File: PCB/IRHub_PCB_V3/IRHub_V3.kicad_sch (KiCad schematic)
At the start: 66 parts, among them J2 USB_C_Receptacle_USB2.0_16P, Q1 UMH3N, Q2 AO3400A, Q3 AO3400A, U1 ESP-12F, U2 CH340C, U3 AMS1117-3.3, U4 TSOP382xx, U5 ME6211C33M5

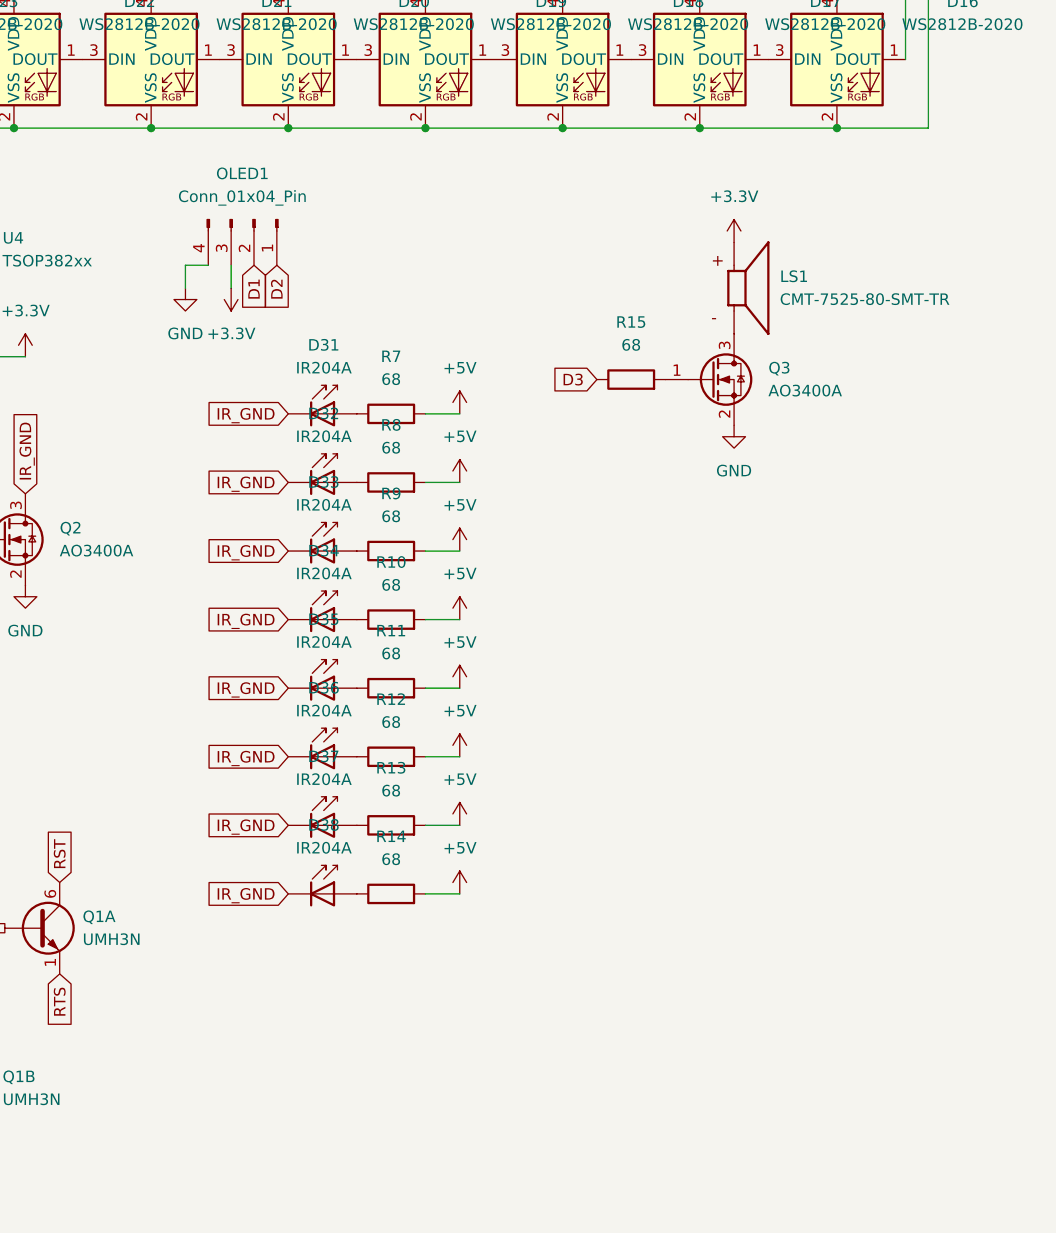
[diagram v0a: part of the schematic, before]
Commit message: complete schematic i think ?
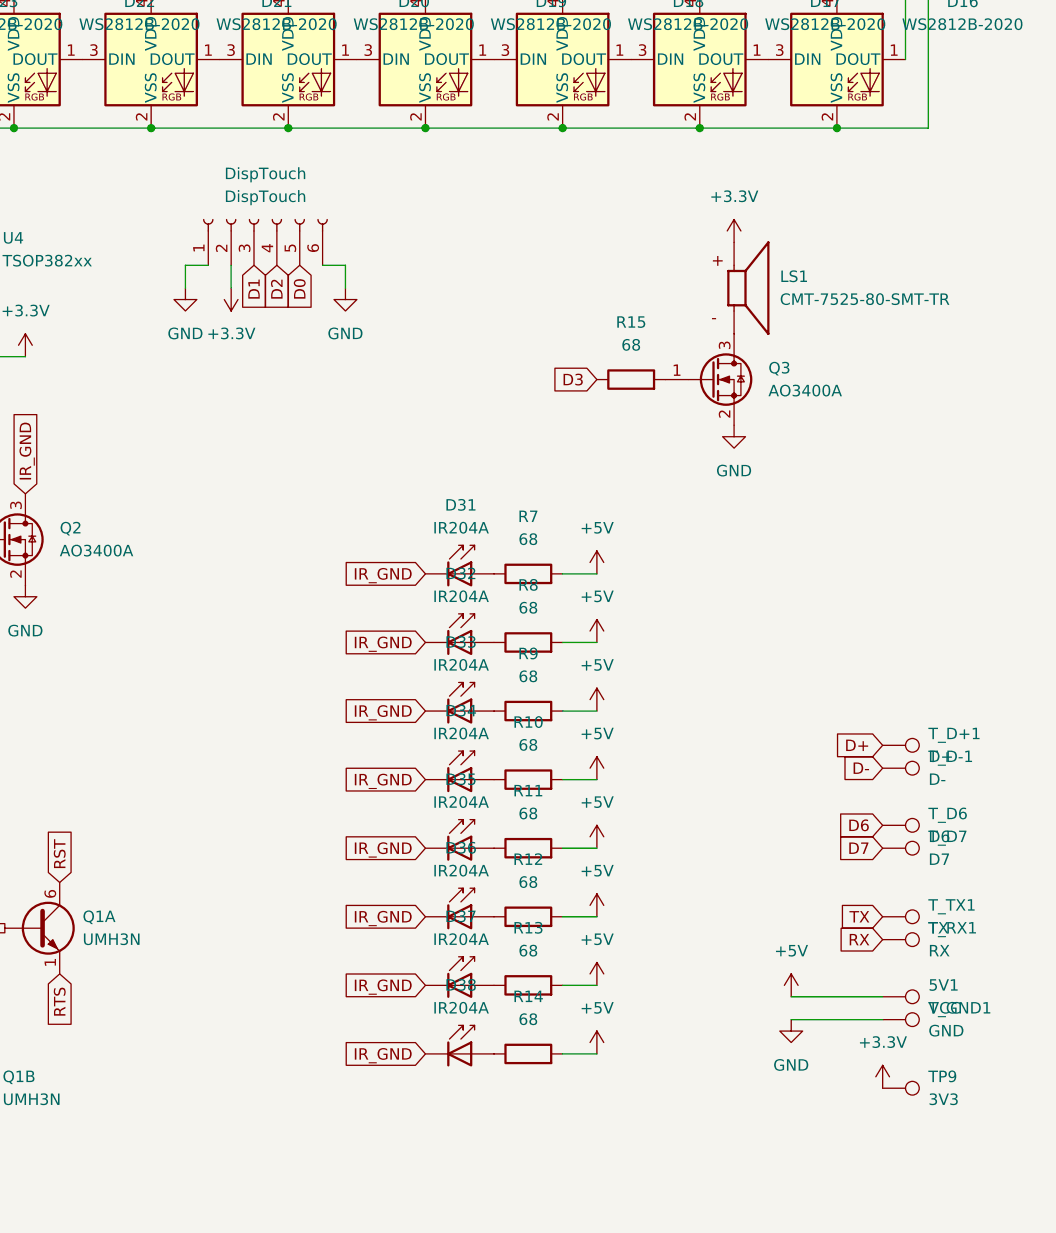
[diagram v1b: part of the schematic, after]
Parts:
- removed OLED1: Conn_01x04_Pin, Connector_PinHeader_2.54mm:PinHeader_1x04_P2.54mm_Vertical, symbol Connector:Conn_01x04_Pin
- added 5V1: VCC, TestPoint:TestPoint_Pad_D2.0mm, symbol Connector:TestPoint
- added DispTouch: DispTouch, Connector_JST:JST_SH_BM06B-SRSS-TB_1x06-1MP_P1.00mm_Vertical, symbol Connector:Conn_01x06_Socket
- added TP9: 3V3, TestPoint:TestPoint_Pad_D2.0mm, symbol Connector:TestPoint
- added T_D+1: D+, TestPoint:TestPoint_Pad_D2.0mm, symbol Connector:TestPoint
- added T_D-1: D-, TestPoint:TestPoint_Pad_D2.0mm, symbol Connector:TestPoint
- added T_D6: D6, TestPoint:TestPoint_Pad_D2.0mm, symbol Connector:TestPoint
- added T_D7: D7, TestPoint:TestPoint_Pad_D2.0mm, symbol Connector:TestPoint
- added T_GND1: GND, TestPoint:TestPoint_Pad_D2.0mm, symbol Connector:TestPoint
- added T_RX1: RX, TestPoint:TestPoint_Pad_D2.0mm, symbol Connector:TestPoint
- added T_TX1: TX, TestPoint:TestPoint_Pad_D2.0mm, symbol Connector:TestPoint
- LS1: footprint CMT-7525-80-SMT-TR:XDCR_CMT-7525-80-SMT-TR -> CMT-7525:XDCR_CMT-7525-80-SMT-TR
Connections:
- net +3.3V: now also DispTouch.2 (Pin_2), TP9.1
- net +5V: now also 5V1.1
- net D+: now also T_D+1.1
- net D-: now also T_D-1.1
- net D0: now also DispTouch.5 (Pin_5)
- net D1: now also DispTouch.3 (Pin_3)
- net D2: now also DispTouch.4 (Pin_4)
- net D6: now also T_D6.1
- net D7: now also T_D7.1
- net GND: now also DispTouch.1 (Pin_1), DispTouch.6 (Pin_6), T_GND1.1
- net RX: now also T_RX1.1
- net TX: now also T_TX1.1
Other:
- moved on the sheet: D31, D32, D33, D34, D35, D36, D37, D38, R10, R11, R12, R13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

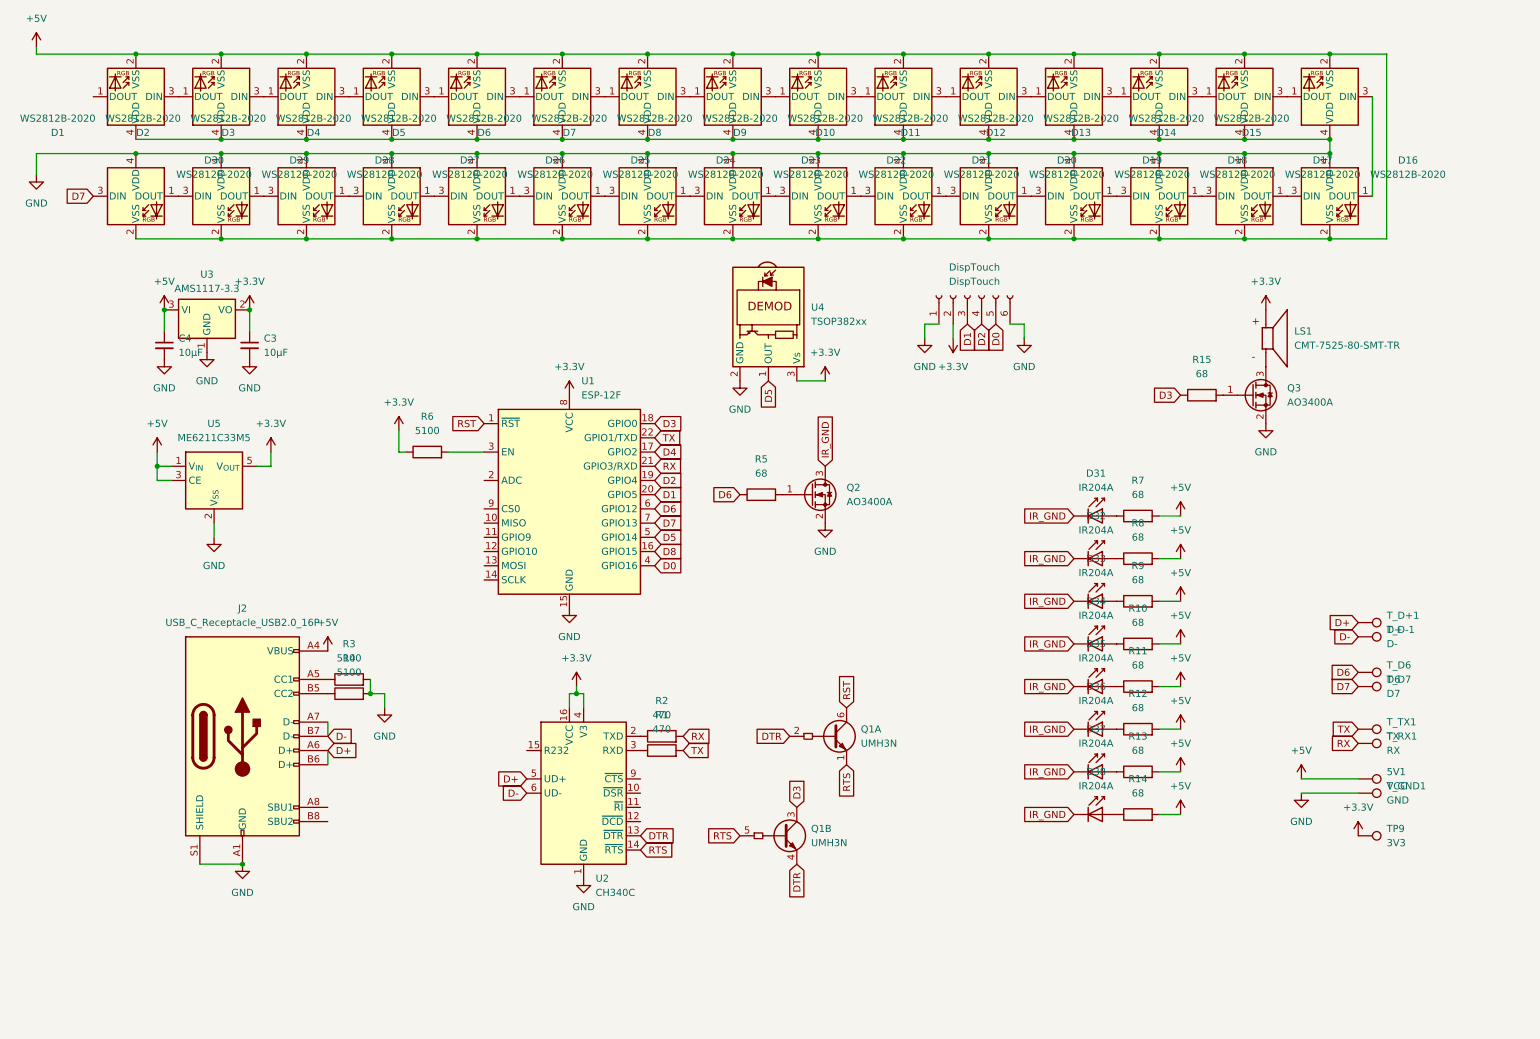
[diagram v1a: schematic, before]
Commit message: final design i think
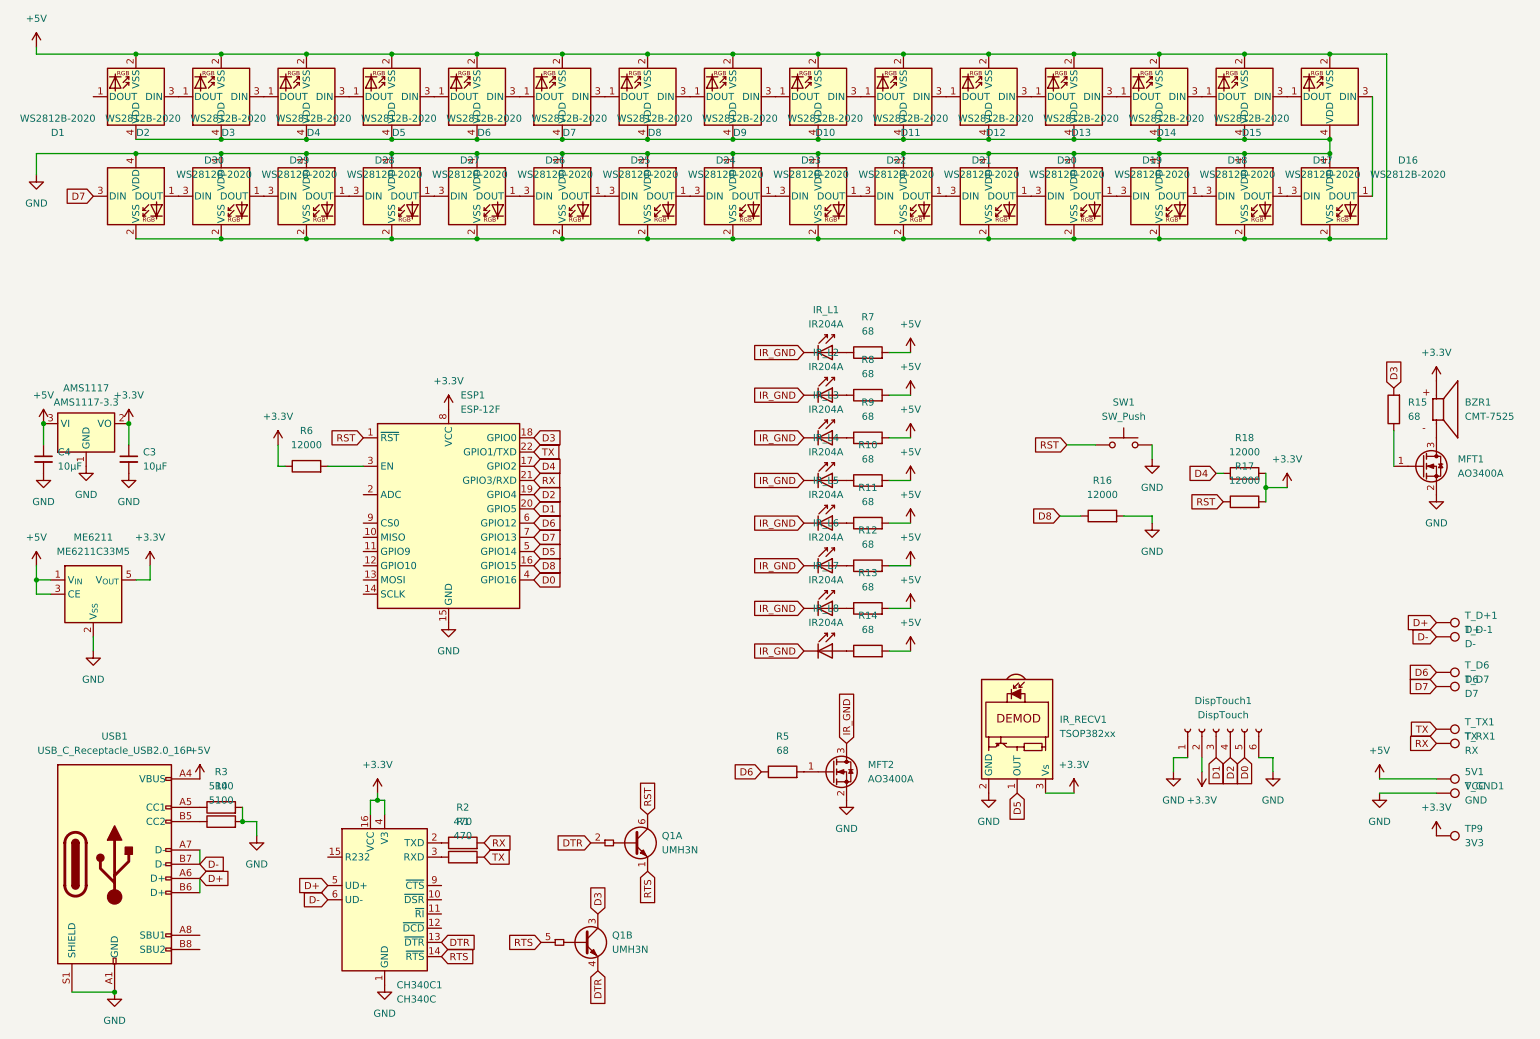
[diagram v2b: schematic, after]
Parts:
- removed D32, D33, D34, D35, D36, D37, D38: IR204A, LED_THT:LED_D3.0mm_IRBlack, symbol LED:IR204A
- added IR_L2, IR_L3, IR_L4, IR_L5, IR_L6, IR_L7, IR_L8: IR204A, LED_THT:LED_D3.0mm_IRBlack, symbol LED:IR204A
- added R16, R17, R18: 12000, Resistor_SMD:R_1206_3216Metric_Pad1.30x1.75mm_HandSolder, symbol Device:R
- added SW1: SW_Push, Button_Switch_SMD:SW_SPST_TS-1088-xR020, symbol Switch:SW_Push
- BZR1: renamed from LS1; value CMT-7525-80-SMT-TR -> CMT-7525
- R6: value 5100 -> 12000
- renumbered U3 to AMS1117, U2 to CH340C1, DispTouch to DispTouch1, U1 to ESP1, D31 to IR_L1, U4 to IR_RECV1, U5 to ME6211, Q3 to MFT1, Q2 to MFT2, J2 to USB1
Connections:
- net +3.3V: now also R17.2, R18.2
- net D3: now also R15.2; no longer R15.1
- net D4: now also R18.1
- net D8: now also R16.1
- net GND: now also R16.2, SW1.2
- net IR_GND: now also IR_L2.1 (K), IR_L3.1 (K), IR_L4.1 (K), IR_L5.1 (K), IR_L6.1 (K), IR_L7.1 (K), IR_L8.1 (K)
- net RST: now also R17.1, SW1.1
- net at R13.1: now also IR_L7.2 (A)
- net at R8.1: now also IR_L2.2 (A)
- net at R11.1: now also IR_L5.2 (A)
- net at R10.1: now also IR_L4.2 (A)
- net at R9.1: now also IR_L3.2 (A)
- net at MFT1.1 (G): now also R15.1; no longer R15.2
- net at R12.1: now also IR_L6.2 (A)
- net at R14.1: now also IR_L8.2 (A)
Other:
- moved on the sheet: 5V1, AMS1117, BZR1, C3, C4, CH340C1, DispTouch1, ESP1, IR_L1, IR_RECV1, ME6211, MFT1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
